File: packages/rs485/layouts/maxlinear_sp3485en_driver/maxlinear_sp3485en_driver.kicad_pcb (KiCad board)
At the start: 2 copper layers, 3 parts

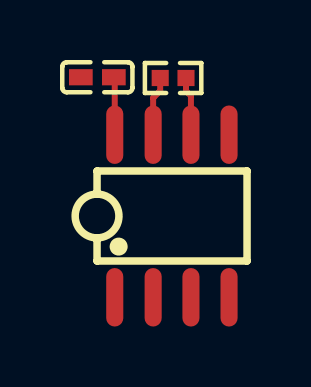
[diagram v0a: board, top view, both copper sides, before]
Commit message: WIP update rs485
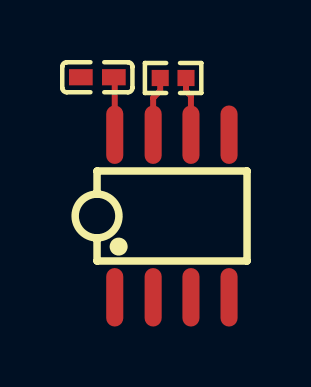
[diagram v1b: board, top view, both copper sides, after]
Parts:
- C1: footprint atopile:C0402-b3ef17 -> Samsung_Electro_Mechanics_CL05B104KO5NNNC:C0402
- R1: footprint atopile:R0402-56259e -> FH_RC_02K1200FT:R0402
- U1: footprint atopile:SOIC-8_L5.0-W4.0-P1.27-LS6.0-BL-294f77 -> MaxLinear_SP3485EN_L_TR:SOIC-8_L5.0-W4.0-P1.27-LS6.0-BL
